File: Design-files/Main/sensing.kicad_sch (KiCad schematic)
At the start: 3 parts, among them U5 AHT21

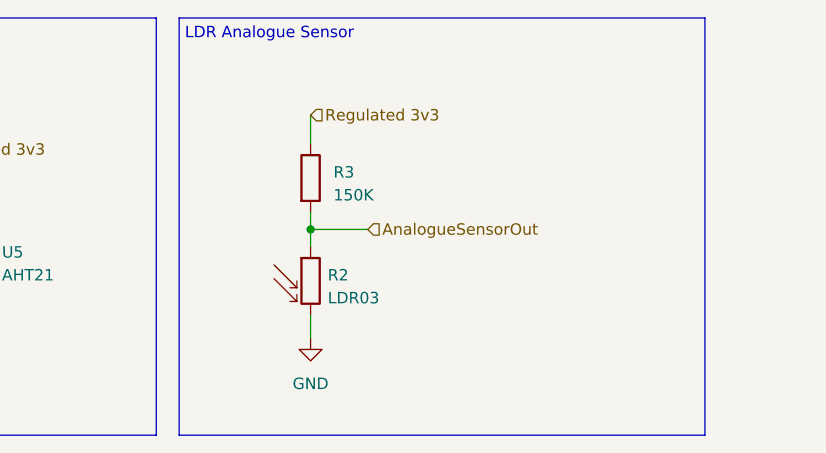
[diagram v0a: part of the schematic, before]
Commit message: Lots of changes :)
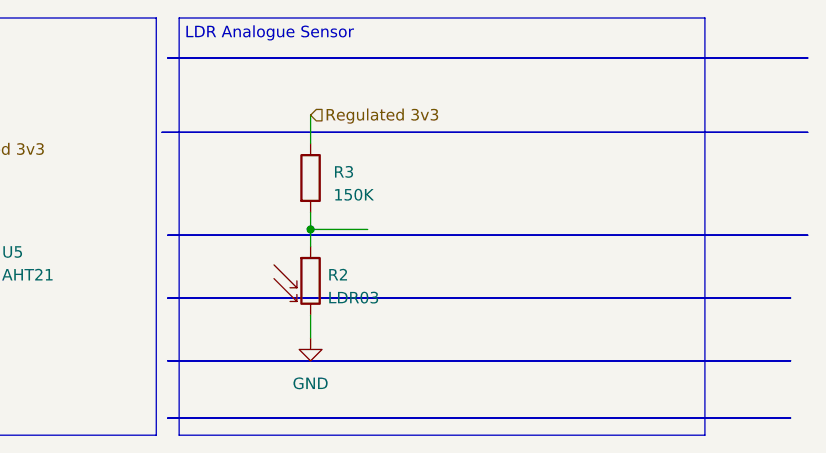
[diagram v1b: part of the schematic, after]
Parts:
- R3: footprint (none) -> Resistor_SMD:R_0201_0603Metric
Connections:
- net AnalogueSensorOut: no longer names the net of R2.1, R3.2
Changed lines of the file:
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@@
     (stroke (width 0) (type default))
+  )
+  (rectangle (start 75.565 53.34) (end 144.78 53.34)
+    (stroke (width 0) (type default))
+    (fill (type none))
+  )
+  (rectangle (start 75.565 46.355) (end 144.78 46.355)
+    (stroke (width 0) (type default))
+    (fill (type none))
   )
   (rectangle (start 14.605 15.24) (end 74.295 61.595)
@@
     (fill (type none))
   )
+  (rectangle (start 75.565 59.69) (end 144.78 59.69)
+    (stroke (width 0) (type default))
+    (fill (type none))
+  )
+  (rectangle (start 75.565 39.37) (end 146.685 39.37)
+    (stroke (width 0) (type default))
+    (fill (type none))
+  )
   (rectangle (start 76.835 15.24) (end 135.255 61.595)
+    (stroke (width 0) (type default))
+    (fill (type none))
+  )
+  (rectangle (start 75.565 19.685) (end 146.685 19.685)
+    (stroke (width 0) (type default))
+    (fill (type none))
+  )
+  (rectangle (start 74.93 27.94) (end 146.685 27.94)
     (stroke (width 0) (type default))
     (fill (type none))
@@
   (hierarchical_label "DigitalSensorSCL" (shape input) (at 34.29 39.37 180) (fields_autoplaced)
     (effects (font (size 1.27 1.27)) (justify right))
-  )
-  (hierarchical_label "AnalogueSensorOut" (shape input) (at 97.79 38.735 0) (fields_autoplaced)
-    (effects (font (size 1.27 1.27)) (justify left))
   )
   (hierarchical_label "Regulated 3v3" (shape input) (at 47.625 29.845 0) (fields_autoplaced)
@@
       (effects (font (size 1.27 1.27)) (justify left))
     )
-    (property "Footprint" "" (at 89.662 33.02 90)
+    (property "Footprint" "Resistor_SMD:R_0201_0603Metric" (at 89.662 33.02 90)
       (effects (font (size 1.27 1.27)) hide)
     )

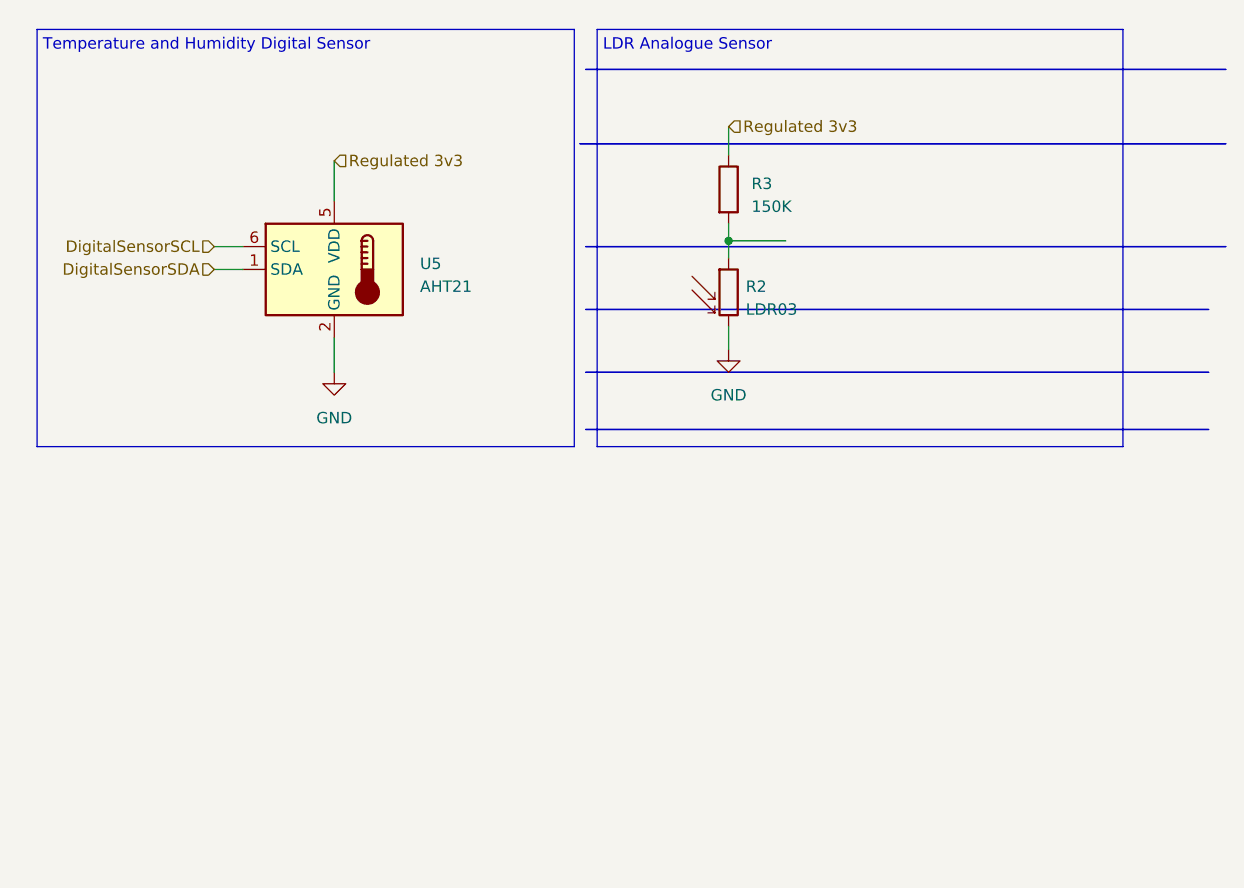
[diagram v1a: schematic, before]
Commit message: changes
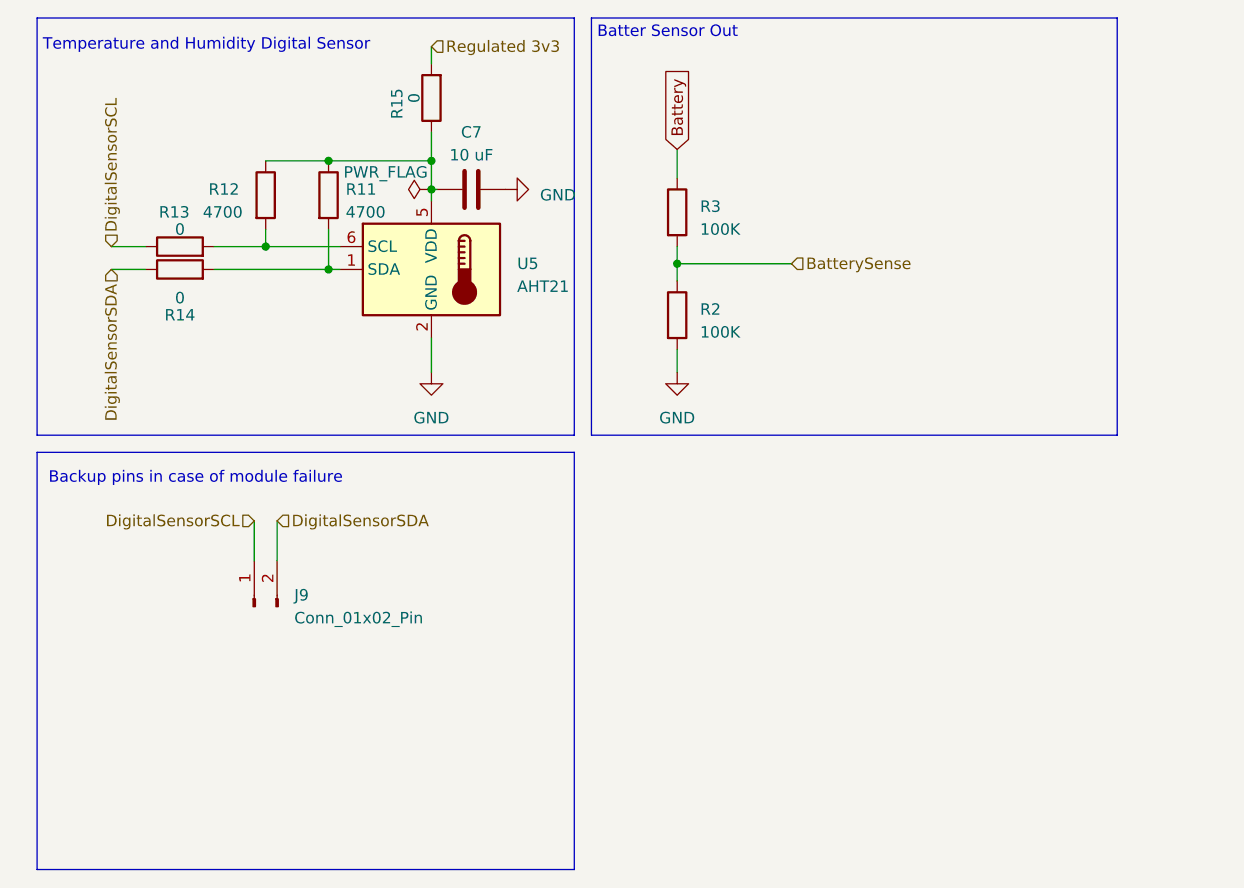
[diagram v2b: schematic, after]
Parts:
- removed R2: LDR03, OptoDevice:R_LDR_10x8.5mm_P7.6mm_Vertical, symbol Sensor_Optical:LDR03
- added C7: 10 uF, symbol Device:C
- added J9: Conn_01x02_Pin, symbol Connector:Conn_01x02_Pin
- added R11, R12: 4700, symbol Device:R
- added R13, R14, R15: 0, symbol Device:R
- added R2: 100K, Resistor_SMD:R_0201_0603Metric, symbol Device:R
- R3: value 150K -> 100K
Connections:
- net DigitalSensorSCL: now also J9.1 (Pin_1), R13.1; no longer U5.6 (SCL)
- net DigitalSensorSDA: now also J9.2 (Pin_2), R14.1; no longer U5.1 (SDA)
- net GND: now also C7.2, R2.2
- net Regulated 3v3: now also R15.2; no longer R3.1, U5.5 (VDD)
- net BatterySense: now reaches R3.2
- net BatterySense: now also R2.1
- new net: C7.1, R11.1, R12.1, R15.1, U5.5 (VDD)
- new net: R12.2, R13.2, U5.6 (SCL)
- new net: R11.2, R14.2, U5.1 (SDA)
- new net Battery: R3.1
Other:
- note added: "Backup pins in case of module failure"
- note added: "Batter Sensor Out"
- note removed: "LDR Analogue Sensor"
- title: (none) -> Sensing Schematic
- moved on the sheet: R3, U5

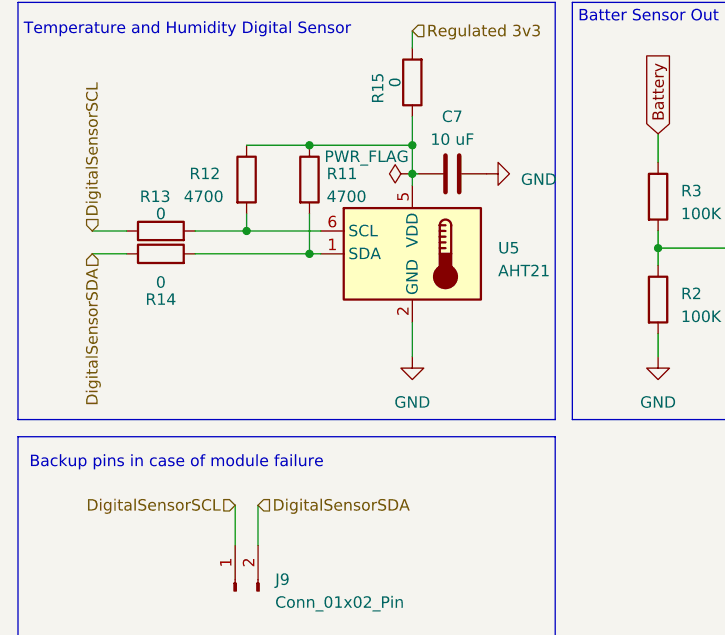
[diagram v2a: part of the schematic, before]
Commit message: changes
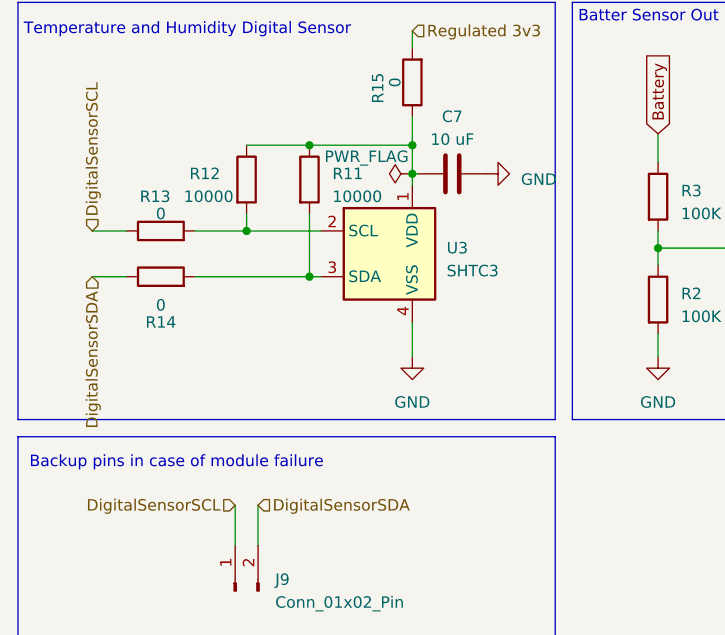
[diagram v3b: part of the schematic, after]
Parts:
- removed U5: AHT21, Package_DFN_QFN:DFN-6-1EP_3x3mm_P1mm_EP1.65x2.55mm, symbol Sensor_Temperature:Si7053-A20
- added U3: SHTC3, Sensor_Humidity:Sensirion_DFN-4-1EP_2x2mm_P1mm_EP0.7x1.6mm, symbol Sensor_Humidity:SHTC3
- C7: footprint (none) -> Capacitor_SMD:C_0201_0603Metric
- J9: footprint (none) -> Connector_PinHeader_2.54mm:PinHeader_1x02_P2.54mm_Vertical
- R11, R12: value 4700 -> 10000; footprint (none) -> Resistor_SMD:R_0201_0603Metric
- R13, R14, R15: footprint (none) -> Resistor_SMD:R_0201_0603Metric
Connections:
- net GND: now also U3.4 (VSS)
- net at C7.1, R11.1, R12.1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: now also U3.1 (VDD)
- net at R12.2, R13.2: now also U3.2 (SCL)
- net at R11.2, R14.2: now also U3.3 (SDA)
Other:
- moved on the sheet: R14

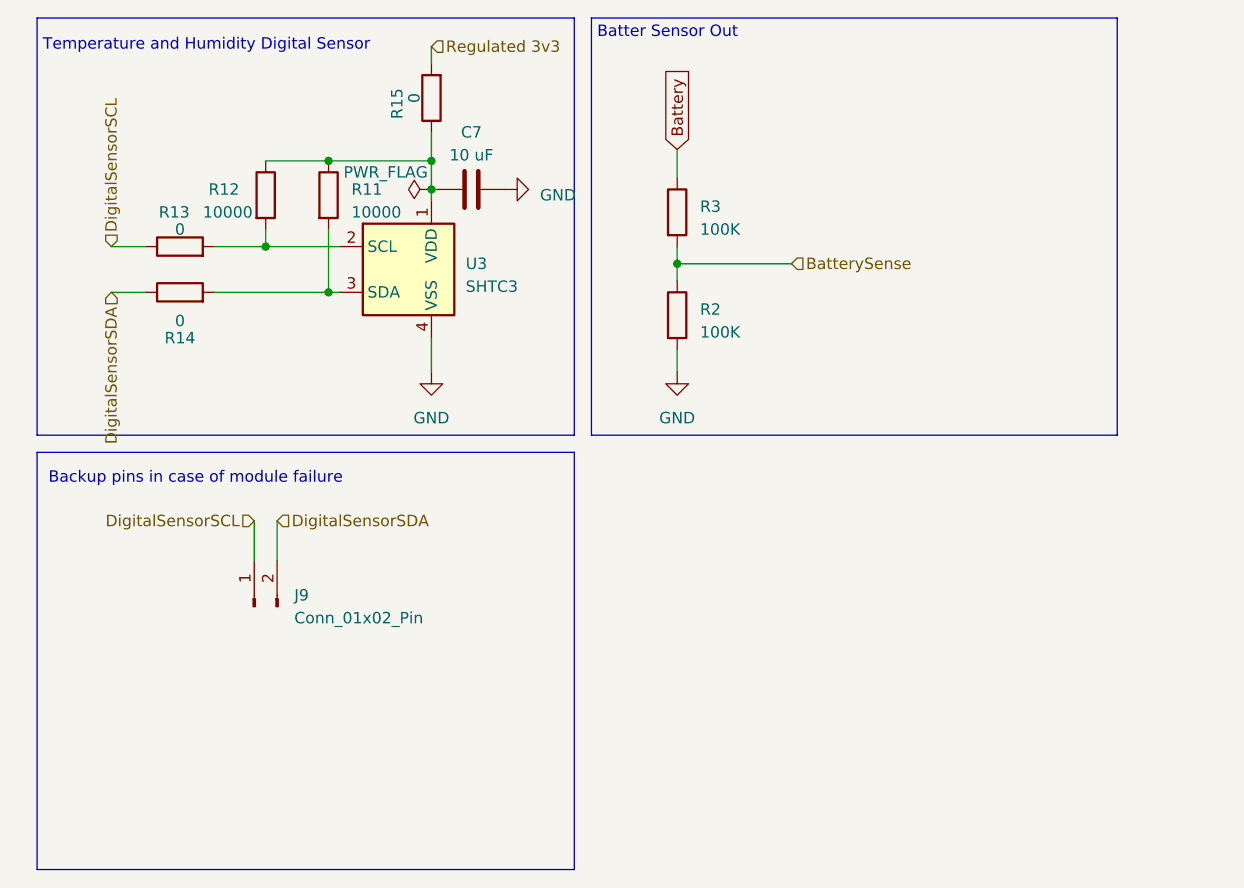
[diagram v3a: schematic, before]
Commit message: lets go team
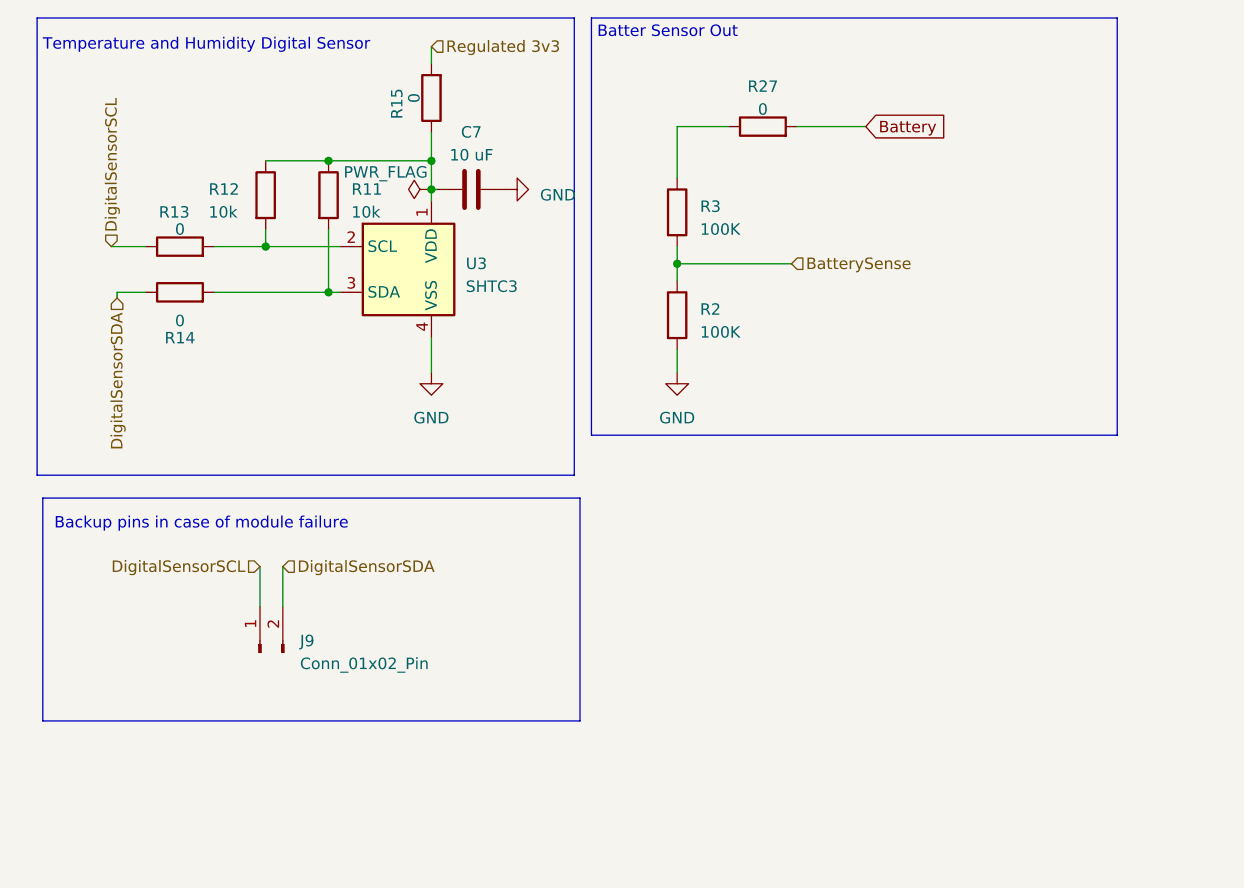
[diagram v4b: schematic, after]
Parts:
- added R27: 0, Resistor_SMD:R_0201_0603Metric, symbol Device:R
- R11, R12: value 10000 -> 10k
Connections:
- net Battery: now also R27.2; no longer R3.1
- new net: R27.1, R3.1
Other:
- moved on the sheet: J9
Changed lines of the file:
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@@
-    (stroke (width 0) (type default))
-  )
-  (wire (pts (xy 85.725 28.575) (xy 85.725 31.75))
     (stroke (width 0) (type default))
   )
@@
     (stroke (width 0) (type default))
   )
-  (wire (pts (xy 22.86 44.45) (xy 26.67 44.45))
-    (stroke (width 0) (type default))
-  )
   (wire (pts (xy 34.29 39.37) (xy 40.005 39.37))
     (stroke (width 0) (type default))
@@
     (stroke (width 0) (type default))
   )
-  (wire (pts (xy 41.275 69.85) (xy 41.275 74.295))
+  (wire (pts (xy 41.91 74.93) (xy 41.91 79.375))
+    (stroke (width 0) (type default))
+  )
+  (wire (pts (xy 99.06 26.035) (xy 106.68 26.035))
     (stroke (width 0) (type default))
   )
@@
     (stroke (width 0) (type default))
   )
+  (wire (pts (xy 23.495 44.45) (xy 26.67 44.45))
+    (stroke (width 0) (type default))
+  )
+  (wire (pts (xy 85.725 26.035) (xy 91.44 26.035))
+    (stroke (width 0) (type default))
+  )
   (wire (pts (xy 85.725 39.37) (xy 85.725 41.275))
     (stroke (width 0) (type default))
@@
     (stroke (width 0) (type default))
   )
-  (wire (pts (xy 38.735 69.85) (xy 38.735 74.295))
+  (wire (pts (xy 39.37 74.93) (xy 39.37 79.375))
+    (stroke (width 0) (type default))
+  )
+  (wire (pts (xy 23.495 45.085) (xy 23.495 44.45))
     (stroke (width 0) (type default))
   )
@@
     (stroke (width 0) (type default))
   )
-  (rectangle (start 14.605 13.97) (end 74.295 60.325)
+  (wire (pts (xy 85.725 26.035) (xy 85.725 31.75))
+    (stroke (width 0) (type default))
+  )
+  (rectangle (start 14.605 13.97) (end 74.295 64.77)
     (stroke (width 0) (type default))
     (fill (type none))
   )
-  (rectangle (start 14.605 62.23) (end 74.295 108.585)
+  (rectangle (start 15.24 67.31) (end 74.93 92.075)
     (stroke (width 0) (type default))
     (fill (type none))
@@
     (fill (type none))
   )
-  (text "Backup pins in case of module failure\n\n" (at 15.875 67.945 0)
+  (text "Backup pins in case of module failure\n\n" (at 16.51 73.025 0)
     (effects (font (size 1.27 1.27)) (justify left bottom))
   )
@@
     (effects (font (size 1.27 1.27)) (justify left bottom))
   )
-  (global_label "Battery" (shape input) (at 85.725 28.575 90) (fields_autoplaced)
-    (effects (font (size 1.27 1.27)) (justify left))
-    (property "Intersheetrefs" "${INTERSHEET_REFS}" (at 85.725 18.9564 90)
+  (global_label "Battery" (shape input) (at 106.68 26.035 0) (fields_autoplaced)
+    (effects (font (size 1.27 1.27)) (justify left))
+    (property "Intersheetrefs" "${INTERSHEET_REFS}" (at 116.2986 26.035 0)
       (effects (font (size 1.27 1.27)) (justify left) hide)
     )
   )
-  (hierarchical_label "DigitalSensorSCL" (shape input) (at 38.735 69.85 180) (fields_autoplaced)
+  (hierarchical_label "DigitalSensorSCL" (shape input) (at 39.37 74.93 180) (fields_autoplaced)
     (effects (font (size 1.27 1.27)) (justify right))
   )
@@
     (effects (font (size 1.27 1.27)) (justify left))
   )
-  (hierarchical_label "DigitalSensorSDA" (shape input) (at 41.275 69.85 0) (fields_autoplaced)
-    (effects (font (size 1.27 1.27)) (justify left))
-  )
-  (hierarchical_label "DigitalSensorSDA" (shape input) (at 22.86 44.45 270) (fields_autoplaced)
+  (hierarchical_label "DigitalSensorSDA" (shape input) (at 41.91 74.93 0) (fields_autoplaced)
+    (effects (font (size 1.27 1.27)) (justify left))
+  )
+  (hierarchical_label "DigitalSensorSDA" (shape input) (at 23.495 45.085 270) (fields_autoplaced)
     (effects (font (size 1.27 1.27)) (justify right))
   )
@@
     )
   )
-  (symbol (lib_id "Connector:Conn_01x02_Pin") (at 38.735 79.375 90) (unit 1)
-    (in_bom yes) (on_board yes) (dnp no) (fields_autoplaced)
-    (property "Reference" "J9" (at 43.18 78.105 90)
+  (symbol (lib_id "Connector:Conn_01x02_Pin") (at 39.37 84.455 90) (unit 1)
+    (in_bom yes) (on_board yes) (dnp no) (fields_autoplaced)
+    (property "Reference" "J9" (at 43.815 83.185 90)
       (effects (font (size 1.27 1.27)) (justify right))
     )
-    (property "Value" "Conn_01x02_Pin" (at 43.18 80.645 90)
+    (property "Value" "Conn_01x02_Pin" (at 43.815 85.725 90)
       (effects (font (size 1.27 1.27)) (justify right))
     )
-    (property "Footprint" "Connector_PinHeader_2.54mm:PinHeader_1x02_P2.54mm_Vertical" (at 38.735 79.375 0)
-      (effects (font (size 1.27 1.27)) hide)
-    )
-    (property "Datasheet" "~" (at 38.735 79.375 0)
+    (property "Footprint" "Connector_PinHeader_2.54mm:PinHeader_1x02_P2.54mm_Vertical" (at 39.37 84.455 0)
+      (effects (font (size 1.27 1.27)) hide)
+    )
+    (property "Datasheet" "~" (at 39.37 84.455 0)
       (effects (font (size 1.27 1.27)) hide)
     )
@@
         (path "/1e9f3d34-a4c0-4684-8b0d-9d61663dabf9/99357ecb-a6bc-4a60-adc8-5fc92399d53b"
           (reference "J9") (unit 1)
+        )
+      )
+    )
+  )
+  (symbol (lib_id "Device:R") (at 95.25 26.035 90) (unit 1)
+    (in_bom yes) (on_board yes) (dnp no) (fields_autoplaced)
+    (property "Reference" "R27" (at 95.25 21.59 90)
+      (effects (font (size 1.27 1.27)))
+    )
+    (property "Value" "0" (at 95.25 24.13 90)
+      (effects (font (size 1.27 1.27)))
+    )
+    (property "Footprint" "Resistor_SMD:R_0201_0603Metric" (at 95.25 27.813 90)
+      (effects (font (size 1.27 1.27)) hide)
+    )
+    (property "Datasheet" "~" (at 95.25 26.035 0)
+      (effects (font (size 1.27 1.27)) hide)
+    )
+    (pin "1")
+    (pin "2")
+    (instances
+      (project "Main"
+        (path "/1e9f3d34-a4c0-4684-8b0d-9d61663dabf9/99357ecb-a6bc-4a60-adc8-5fc92399d53b"
+          (reference "R27") (unit 1)
         )
       )
@@
       (effects (font (size 1.27 1.27)) (justify left))
     )
-    (property "Value" "10000" (at 33.02 35.56 0)
+    (property "Value" "10k" (at 33.655 35.56 0)
       (effects (font (size 1.27 1.27)) (justify left))
     )
@@
       (effects (font (size 1.27 1.27)) (justify left))
     )
-    (property "Value" "10000" (at 49.53 35.56 0)
-      (effects (font (size 1.27 1.27)) (justify left))
-    )
+    (property "Value" "10k" (at 49.53 35.56 0)
+      (effects (font (size 1.27 1.27)) (justify left))
+    )
